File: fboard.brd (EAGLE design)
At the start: 60.9 x 51.7 mm, 29 parts, among them Q1 SL2305, U1 ATMEGA328PB-AU, U2 MPU-6050, U3 SN74HC138PW

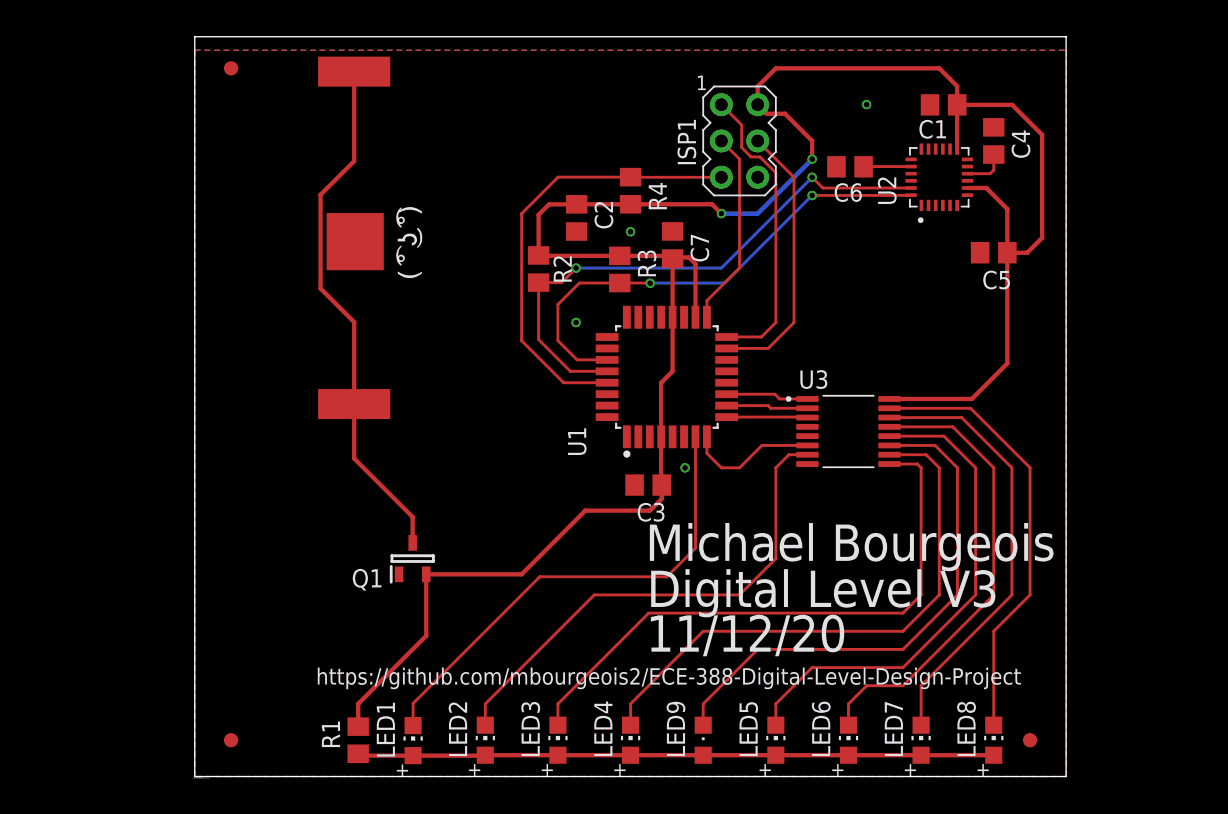
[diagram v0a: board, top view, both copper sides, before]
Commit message: ground plane?
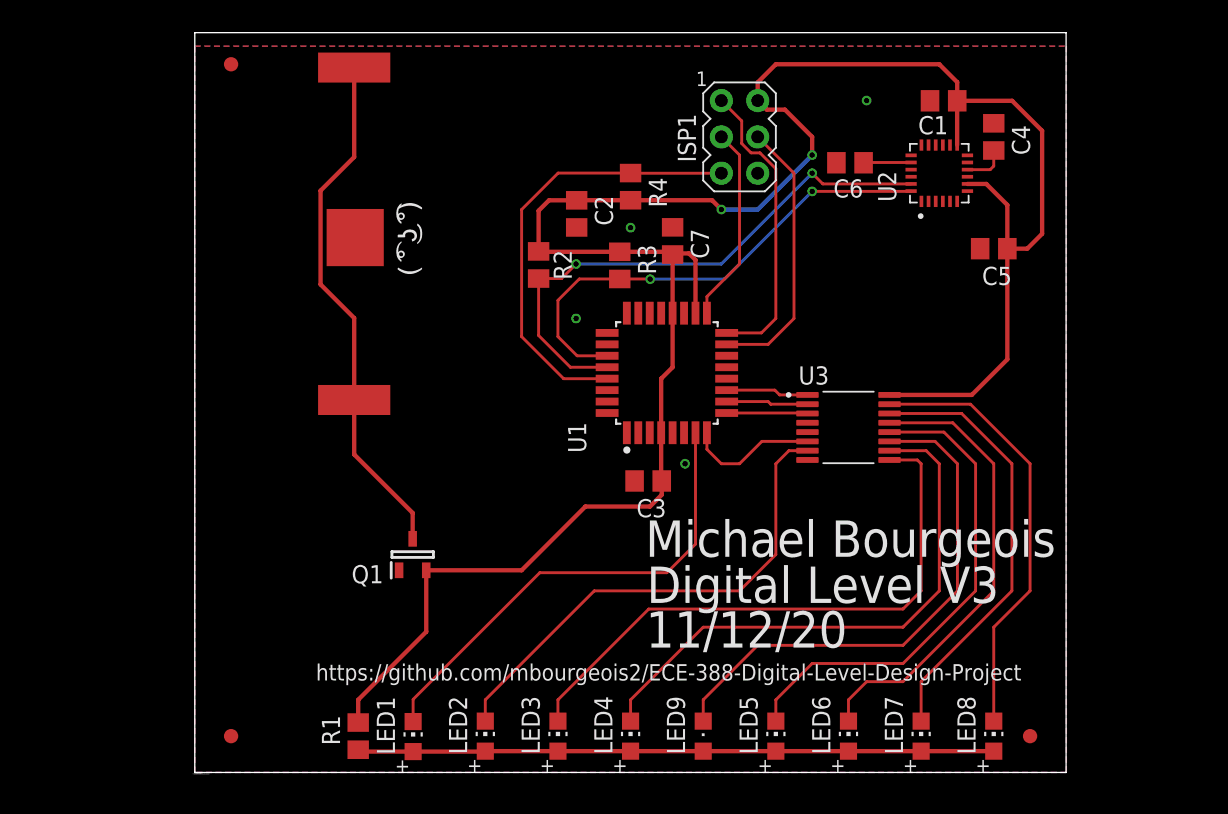
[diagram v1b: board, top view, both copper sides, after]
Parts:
- moved U2 0.28 mm to (52.2, 42.2)
- moved LED1 0.28 mm to (15.4, 2.79)
- moved LED2 0.28 mm to (20.5, 2.82)
- moved LED3 0.28 mm to (25.5, 2.82)
- moved LED4 0.28 mm to (30.6, 2.82)
- moved LED5 0.28 mm to (40.8, 2.82)
- moved LED6 0.28 mm to (45.9, 2.82)
- moved LED7 0.28 mm to (50.9, 2.82)
- moved LED8 0.28 mm to (56.0, 2.82)
- moved LED9 0.28 mm to (35.7, 2.82)
- moved R1 0.28 mm to (11.6, 2.82)
- moved U$4 0.28 mm to (58.6, 2.82)
- moved U$6 0.28 mm to (2.68, 2.82)
- moved BAT1 0.28 mm to (7.76, 48.5)
- moved C1 0.28 mm to (52.5, 47.3)
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
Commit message: fixed airwire
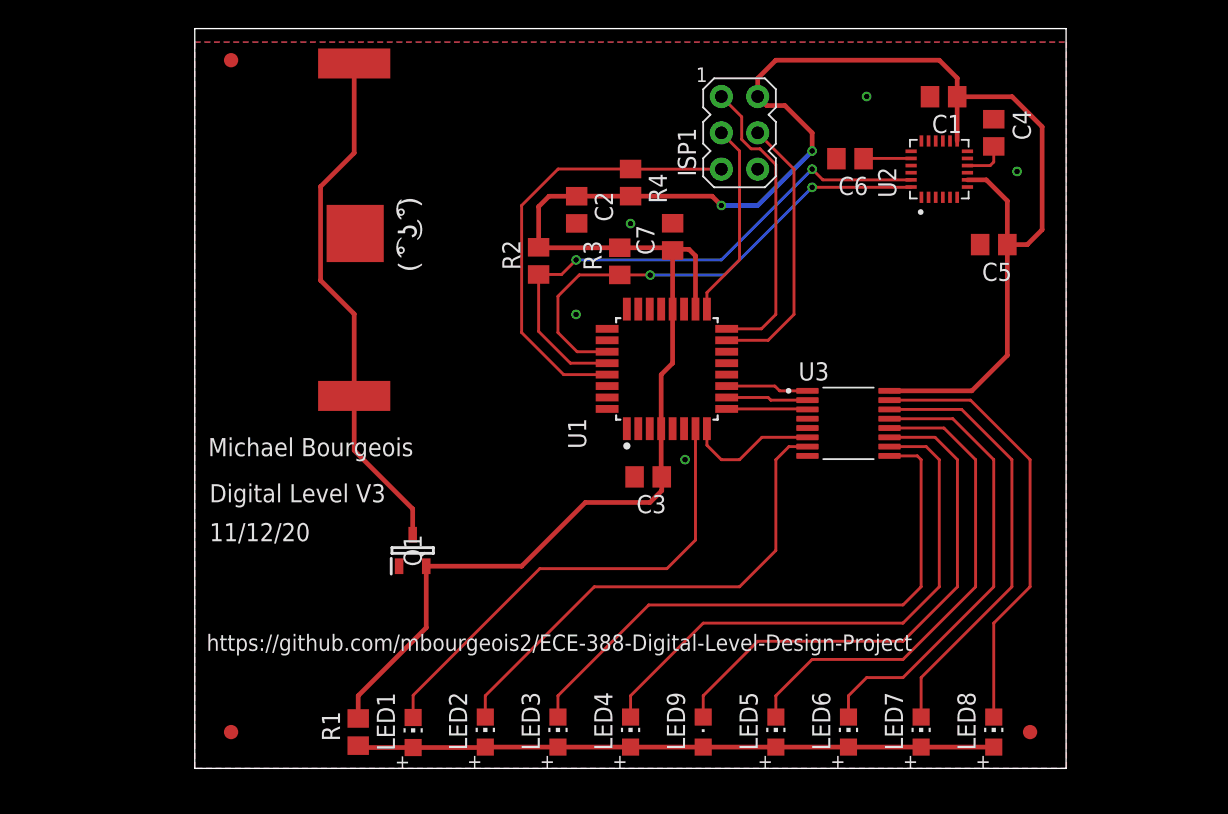
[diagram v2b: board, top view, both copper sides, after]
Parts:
- moved C2 0.28 mm to (26.9, 39.6)
- moved U3 0.28 mm to (45.9, 24.7)
- moved Q1 0.28 mm to (15.4, 15.8)
- moved LED1 0.28 mm to (15.4, 3.08)
- moved LED2 0.28 mm to (20.5, 3.11)
- moved LED3 0.28 mm to (25.5, 3.11)
- moved LED4 0.28 mm to (30.6, 3.11)
- moved LED5 0.28 mm to (40.8, 3.11)
- moved LED6 0.28 mm to (45.9, 3.11)
- moved LED7 0.28 mm to (50.9, 3.11)
- moved LED8 0.28 mm to (56.0, 3.11)
- moved LED9 0.28 mm to (35.7, 3.11)
- moved R1 0.28 mm to (11.6, 3.11)
- moved U$4 0.28 mm to (58.6, 3.11)
- moved U$6 0.28 mm to (2.68, 3.11)
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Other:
- board text removed: "C:/Users/Michael/Desktop/lenny.bmp"
